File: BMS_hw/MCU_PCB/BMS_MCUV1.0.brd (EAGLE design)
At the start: 60 x 30 mm, 42 parts, among them IC2 SST25VF020B804ISA, Q1 CRYSTALS-GND-LID-IQXC-42

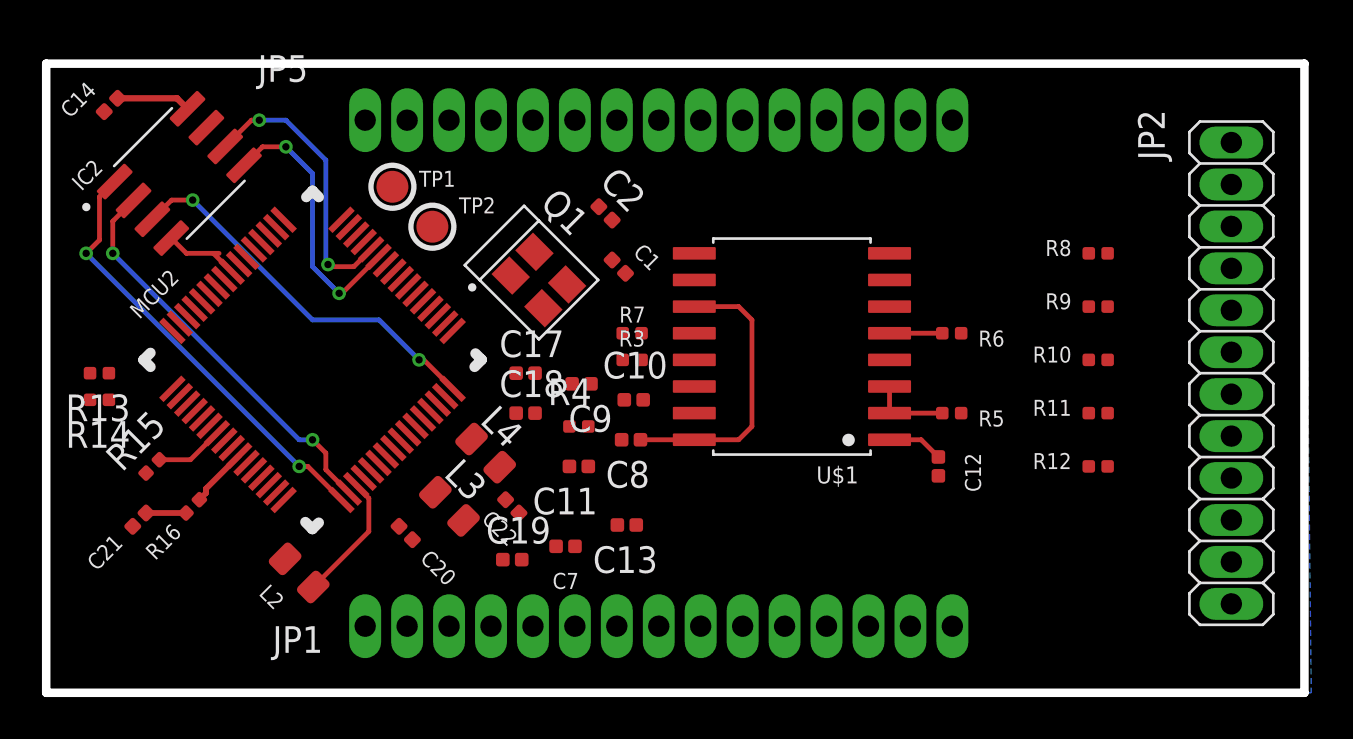
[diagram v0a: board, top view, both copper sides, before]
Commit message: brd layout and sch update @14
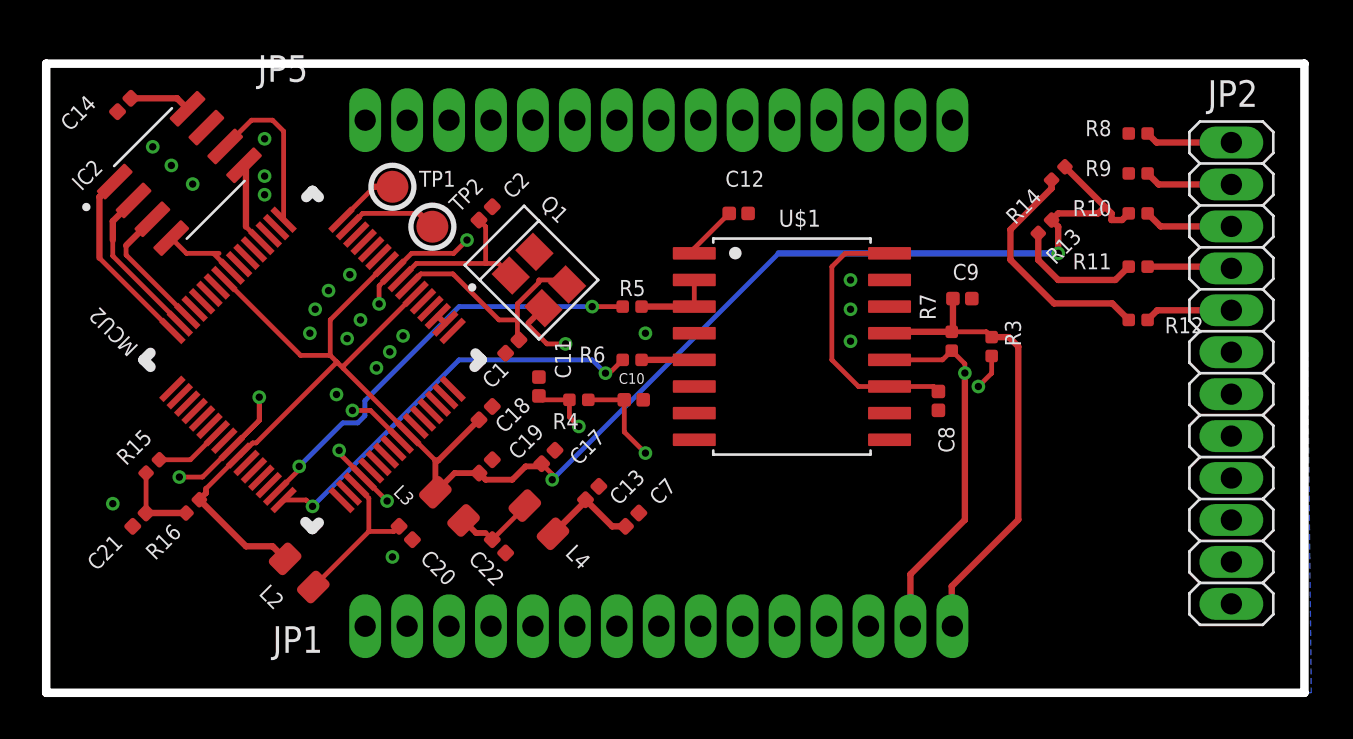
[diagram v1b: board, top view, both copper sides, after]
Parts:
- moved R14 47.0 mm to (48.3, 24.8), turned to 225 degrees
- moved R13 45.6 mm to (47.6, 22.2), turned to 225 degrees
- moved C9 18.6 mm to (43.7, 18.8), turned to 0 degrees
- moved R3 17.2 mm to (45.1, 16.5), turned to 270 degrees
- moved R5 16.1 mm to (27.9, 18.4), turned to 0 degrees
- moved C12 15.4 mm to (33.0, 22.9), turned to 0 degrees
- moved R6 15.3 mm to (27.9, 15.9), turned to 0 degrees
- moved R7 15.2 mm to (43.2, 16.8), turned to 90 degrees
- moved C8 14.8 mm to (42.5, 13.9), turned to 270 degrees
- moved R12 7.24 mm to (52.1, 17.8), turned to 0 degrees
- moved R10 7.24 mm to (52.1, 22.9), turned to 0 degrees
- moved R11 7.24 mm to (52.1, 20.3), turned to 0 degrees
- moved R9 6.63 mm to (52.1, 24.8), turned to 0 degrees
- moved C1 6.35 mm to (22.2, 16.5), turned to 225 degrees
- moved R8 6.02 mm to (52.1, 26.7), turned to 0 degrees
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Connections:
- removed net DBG_RX: MCU2.64
- removed net INTL_OUT: MCU2.49
- removed net N$68: MCU2.62
- removed net N$69: MCU2.63
- removed net N$76: MCU2.52
- new net N$12: JP2.10, R10.2
- new net N$13: JP2.9, R11.2
- new net N$15: JP2.8, R12.2
- new net N$4: JP2.12, R8.2
- new net N$8: JP2.11, R9.2
- net CANH: now also JP1.15
- net CANL: now also JP1.14
- net CE#: now also MCU2.64; no longer MCU2.17
- net SCK: now also MCU2.49; no longer MCU2.44
- net SI: now also MCU2.52; no longer MCU2.43
- net SO: now also MCU2.63; no longer MCU2.18
- net WP#: now also MCU2.62; no longer MCU2.32
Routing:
- net VDD: track 2.89 -> 87.6 mm, vias 0 -> 2
- net CANL: track 0.00 -> 39.1 mm, vias 0 -> 2
- net N$11: track 0.00 -> 24.5 mm, vias 0 -> 2
- net GND: track 3.82 -> 28.3 mm, vias 0 -> 30
- net CANH: track 0.00 -> 22.7 mm
- net CAN_RX: track 0.00 -> 20.7 mm, vias 0 -> 2
- net CAN_TX: track 0.00 -> 19.7 mm, vias 0 -> 2
- net CE#: track 21.0 -> 8.86 mm, vias 2 -> 0
- net WP#: track 18.4 -> 6.35 mm, vias 2 -> 0
- net SO: track 19.4 -> 7.60 mm, vias 2 -> 0
- net SCL: track 0.00 -> 11.4 mm
- net N$1: track 0.00 -> 11.1 mm
- net SI: track 13.0 -> 4.00 mm, vias 2 -> 0
- net N$2: track 0.00 -> 7.99 mm
- net SDA: track 0.00 -> 6.24 mm
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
